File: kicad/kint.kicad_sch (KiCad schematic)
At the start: 25 parts, among them J1 THUMB_RIGHT_SPC_KB600, J2 LEFT_13_LT, J3 TOP_LEFT, J4 TOP_RIGHT, J5 THUMB_LEFT_BAK, J6 THUMB_RIGHT_SPC, J7 RIGHT_13_DOWN, J8 THUMB_LEFT_BAK_KB600, U1 TEENSY_3.5_3.6

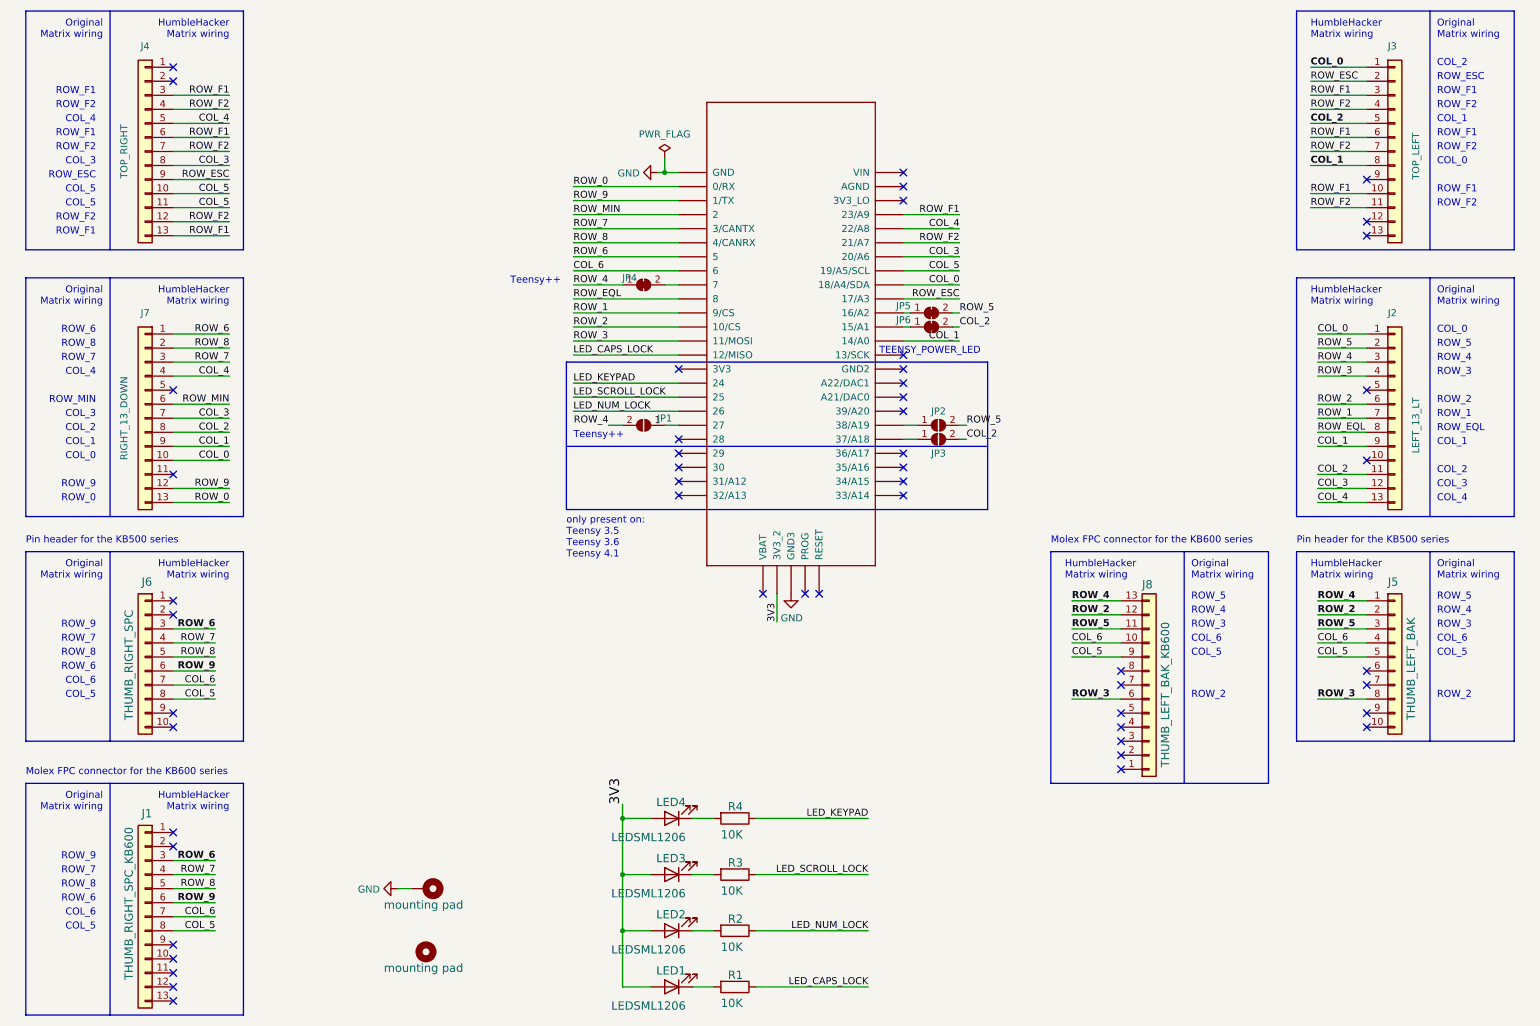
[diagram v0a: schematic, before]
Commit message: [WIP] playing around with promicro compatibility
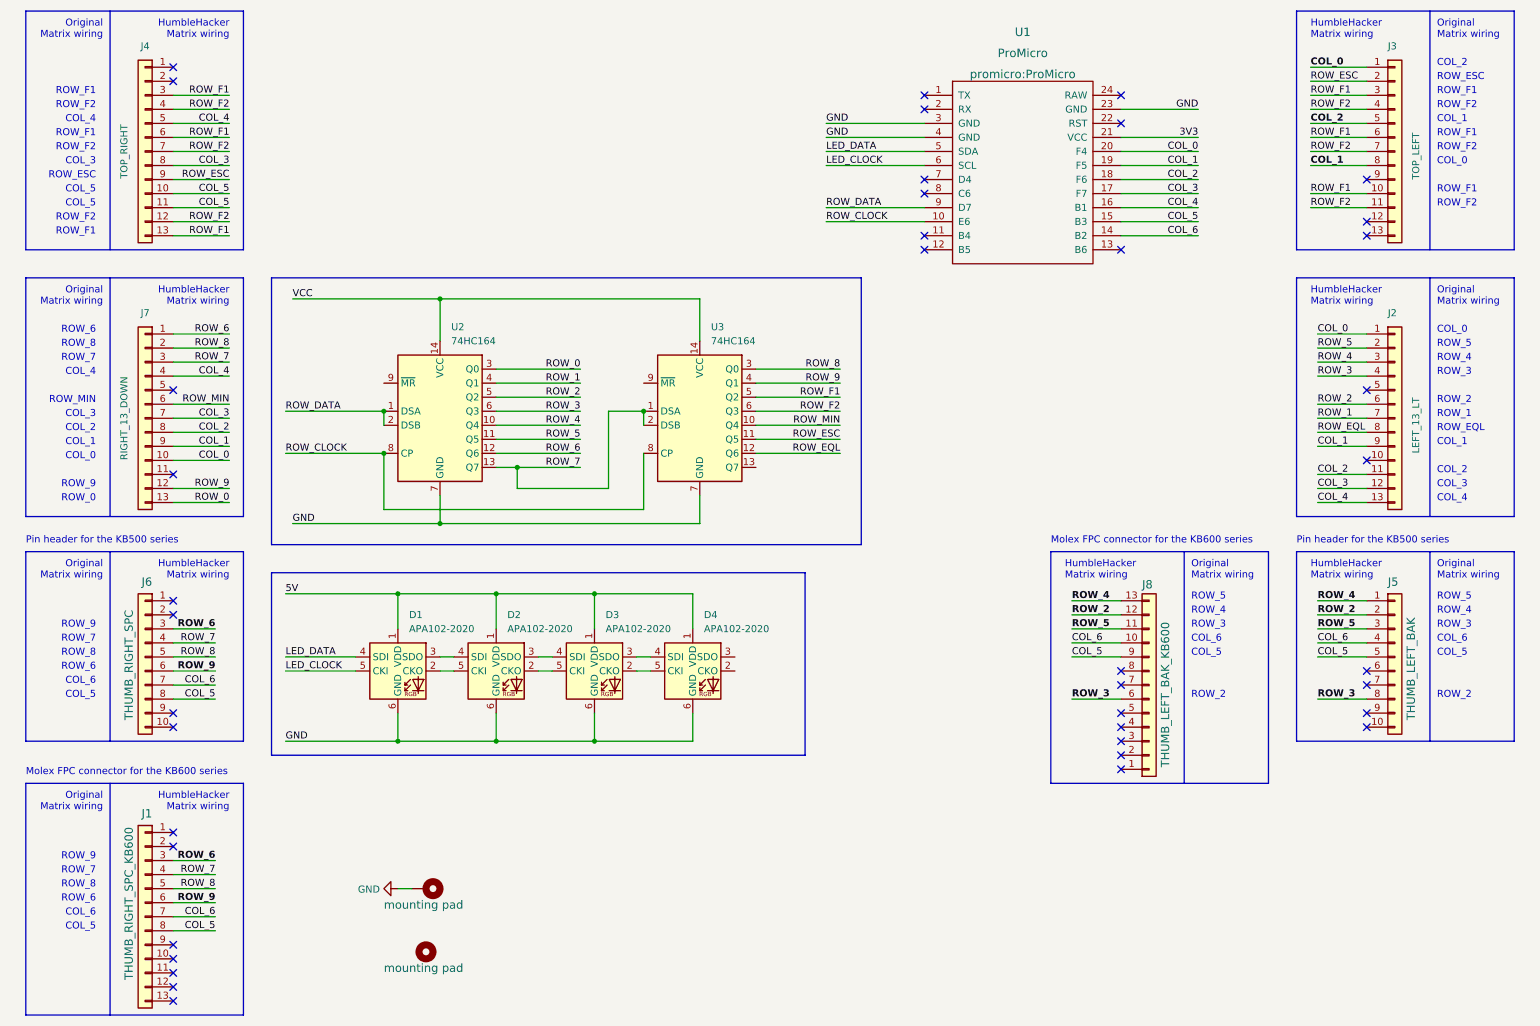
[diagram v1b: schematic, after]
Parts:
- removed JP1, JP2, JP3: SolderJumper_2_Open, Jumper:SolderJumper-2_P1.3mm_Open_RoundedPad1.0x1.5mm, symbol Jumper:SolderJumper_2_Open
- removed JP4, JP5, JP6: SolderJumper_2_Bridged, Jumper:SolderJumper-2_P1.3mm_Bridged2Bar_RoundedPad1.0x1.5mm, symbol Jumper:SolderJumper_2_Bridged
- removed LED1, LED2, LED3, LED4: LEDSML1206, LED_SMD:LED_1206_3216Metric_Pad1.42x1.75mm_HandSolder, symbol Device:LED
- removed R1, R2, R3, R4: 10K, Resistor_SMD:R_1206_3216Metric_Pad1.42x1.75mm_HandSolder, symbol Device:R
- removed U1: TEENSY_3.5_3.6, kinx:TEENSY_3.5_3.6, symbol kinx-eagle-import:TEENSY_3.5_3.6
- added D1, D2, D3, D4: APA102-2020, LED_SMD:LED-APA102-2020, symbol LED:APA102-2020
- added U1: ProMicro, promicro:ProMicro, symbol ProMicroKiCad:ProMicro
- added U2, U3: 74HC164, Package_SO:TSSOP-14_4.4x5mm_P0.65mm, symbol 74xx:74HC164
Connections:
- net 3V3: now also U1.21 (VCC)
- net COL_0: now also U1.20 (F4)
- net COL_1: now also U1.19 (F5)
- net COL_2: now also U1.18 (F6)
- net COL_3: now also U1.17 (F7)
- net COL_4: now also U1.16 (B1)
- net COL_5: now also U1.15 (B3)
- net COL_6: now also U1.14 (B2)
- net GND: now also D1.6 (GND), D2.6 (GND), D3.6 (GND), D4.6 (GND), U1.23 (GND), U1.3 (GND), U1.4 (GND), U2.7 (GND), U3.7 (GND)
- net ROW_0: now also U2.3 (Q0)
- net ROW_1: now also U2.4 (Q1)
- net ROW_2: now also U2.5 (Q2)
- net ROW_3: now also U2.6 (Q3)
- net ROW_4: now also U2.10 (Q4)
- net ROW_5: now also U2.11 (Q5)
- net ROW_6: now also U2.12 (Q6)
- net ROW_7: now also U2.13 (Q7), U3.1 (DSA), U3.2 (DSB)
- net ROW_8: now also U3.3 (Q0)
- net ROW_9: now also U3.4 (Q1)
- net ROW_EQL: now also U3.12 (Q6)
- net ROW_ESC: now also U3.11 (Q5)
- net ROW_F1: now also U3.5 (Q2)
- net ROW_F2: now also U3.6 (Q3)
- net ROW_MIN: now also U3.10 (Q4)
- new net: D3.3 (SDO), D4.4 (SDI)
- new net: D3.2 (CKO), D4.5 (CKI)
- new net: D2.2 (CKO), D3.5 (CKI)
- new net: D2.3 (SDO), D3.4 (SDI)
- new net: D1.3 (SDO), D2.4 (SDI)
- new net: D1.2 (CKO), D2.5 (CKI)
- new net 5V: D1.1 (VDD), D2.1 (VDD), D3.1 (VDD), D4.1 (VDD)
- new net LED_CLOCK: D1.5 (CKI), U1.6 (SCL)
- new net LED_DATA: D1.4 (SDI), U1.5 (SDA)
- new net ROW_CLOCK: U1.10 (E6), U2.8 (CP), U3.8 (CP)
- new net ROW_DATA: U1.9 (D7), U2.1 (DSA), U2.2 (DSB)
- new net VCC: U2.14 (VCC), U3.14 (VCC)
- no-connect marks 52 -> 40
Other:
- note removed: "TEENSY_POWER_LED"
- note removed: "Teensy++"
- note removed: "only present on: Teensy 3.5 Teensy 3.6 Teensy 4.1"
